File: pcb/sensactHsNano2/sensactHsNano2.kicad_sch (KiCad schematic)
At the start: 64 parts, among them J1 PROG, J2 SensactBusConnector, J3 CAN+24V, J5 Audio, J6 Conn_01x03, J8 Conn_01x10, SW1 TERM ON, SW2 Prog, SW3 Reset, SW4 PROG_PWR, U10 ADS1115IDGS, U11 L78L15_SOT89, U12 SRV05, U3 ESP32, U4 DS2482, U5 SN65HVD230, U8 LM358, U9 MCP4728

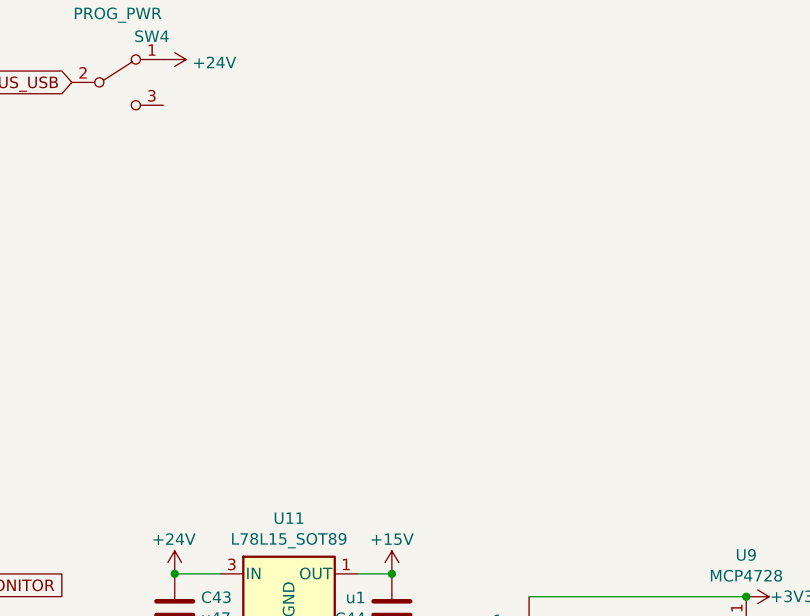
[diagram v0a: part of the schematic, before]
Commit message: Sicherung
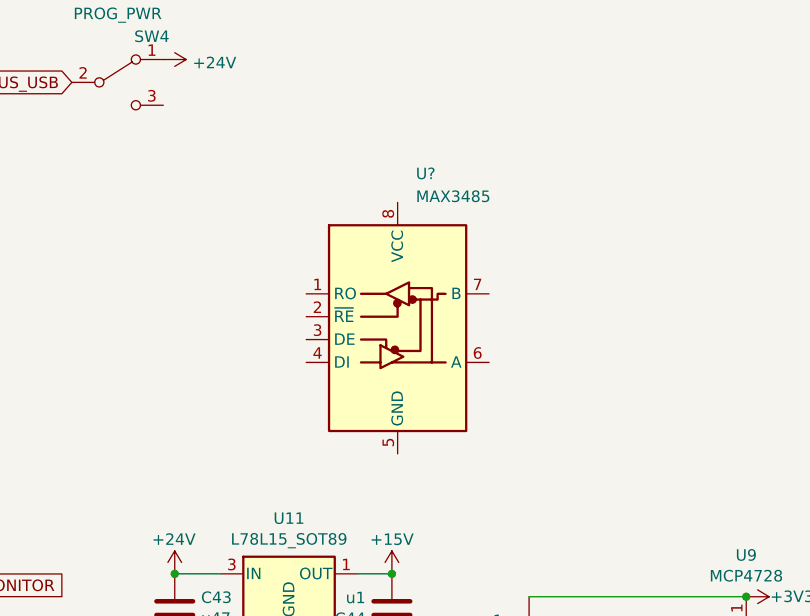
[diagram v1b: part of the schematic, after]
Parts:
- added U?: MAX3485, symbol Interface_UART:MAX3485
